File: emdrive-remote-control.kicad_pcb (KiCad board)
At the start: 2 copper layers, 107 x 46 mm, 43 parts, among them J1 Raspberry_Pi_2_3, J2 Screw_Terminal_01x06, J3 Conn_01x04, K1 Relay_SPST-NO, Q1 DMN61D8LQ, SW3 SW_Push, SW4 SW_Push, U1 ADS1015IDGS, U2 WS2801SO, U3 AP62150WU, U5 SN74HCS125, U6 MCP602, U7 BTS6143D

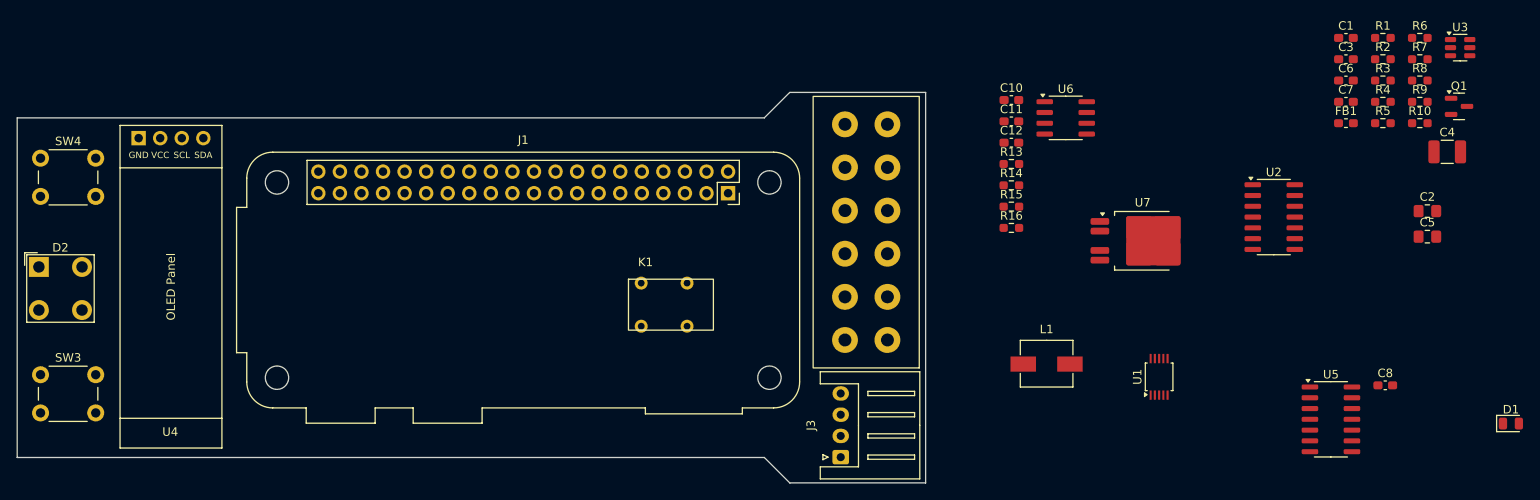
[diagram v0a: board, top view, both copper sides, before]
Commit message: Continues SCH, placed components on PCB
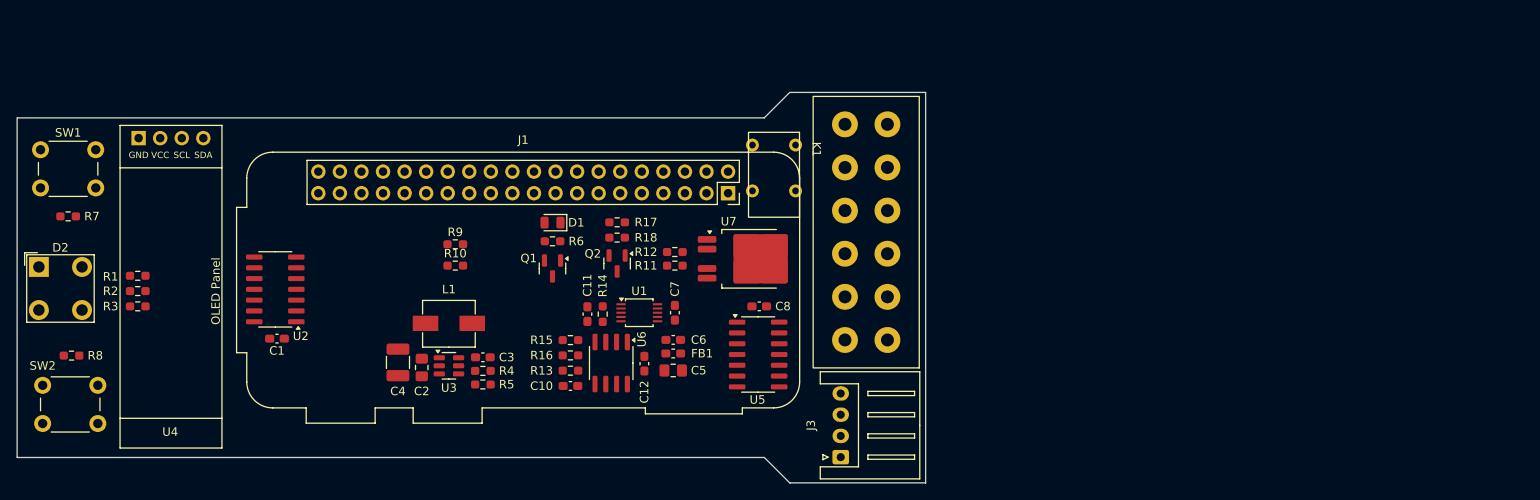
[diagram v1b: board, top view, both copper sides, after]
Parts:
- removed SW3, SW4: SW_Push, Button_Switch_THT:SW_PUSH_6mm_H8mm
- added Q2: MMBT3904, Package_TO_SOT_SMD:SOT-23, F.Cu at (149.7, 67.2)
- added R11: 33k, Resistor_SMD:R_0603_1608Metric_Pad0.98x0.95mm_HandSolder, F.Cu at (156.5, 67.4)
- added R12: 33k, Resistor_SMD:R_0603_1608Metric_Pad0.98x0.95mm_HandSolder, F.Cu at (156.5, 65.8)
- added R17: 33k, Resistor_SMD:R_0603_1608Metric_Pad0.98x0.95mm_HandSolder, F.Cu at (149.7, 62.3)
- added R18: 33k, Resistor_SMD:R_0603_1608Metric_Pad0.98x0.95mm_HandSolder, F.Cu at (149.7, 64.1)
- added SW1: SW_Push, Button_Switch_THT:SW_PUSH_6mm_H8mm, F.Cu at (81.8, 53.8)
- added SW2: SW_Push, Button_Switch_THT:SW_PUSH_6mm_H8mm, F.Cu at (82.0, 81.5)
- moved R8 162.1 mm to (85.4, 78.0)
- moved R7 160.3 mm to (85.0, 61.6)
- moved R1 149.3 mm to (93.2, 68.6), turned to 180 degrees
- moved R2 149.2 mm to (93.2, 70.4), turned to 180 degrees
- moved R3 149.1 mm to (93.2, 72.2), turned to 180 degrees
- moved C1 130.8 mm to (109.6, 76.0), turned to 180 degrees
- moved C4 126.1 mm to (123.8, 78.8), turned to 90 degrees
- moved U3 124.9 mm to (129.8, 79.2)
- moved C2 119.9 mm to (126.7, 79.4), turned to -90 degrees
- moved U2 117.9 mm to (109.4, 70.2), turned to 180 degrees
- moved D1 115.3 mm to (142.1, 62.3), turned to 180 degrees
- moved R10 114.8 mm to (130.6, 67.4)
- moved R9 114.8 mm to (130.6, 64.9)
- moved R4 110.6 mm to (133.8, 79.8), turned to 180 degrees
- moved R5 110.4 mm to (133.8, 81.4)
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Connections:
- C10 pad 1: GNDA -> GND
- C11 pad 1: GNDA -> GND
- C12 pad 1: GNDA -> GND
- C6 pad 1: GNDA -> GND
- J1 pad 1: Net-(J1-3V3-Pad1) -> +3.3V
- J1 pad 14: Net-(J1-GND-Pad14) -> GND
- J1 pad 15: unconnected-(J1-GPIO22-Pad15) -> /IN_LED_R
- J1 pad 16: unconnected-(J1-GPIO23-Pad16) -> /IN_LED_G
- J1 pad 17: Net-(J1-3V3-Pad1) -> +3.3V
- J1 pad 18: unconnected-(J1-GPIO24-Pad18) -> /IN_LED_Y
- J1 pad 19: unconnected-(J1-MOSI0/GPIO10-Pad19) -> /SPI_MOSI
- J1 pad 2: Net-(J1-5V-Pad2) -> +5V
- J1 pad 20: Net-(J1-GND-Pad14) -> GND
- J1 pad 23: unconnected-(J1-SCLK0/GPIO11-Pad23) -> /SPI_SCLK
- J1 pad 25: Net-(J1-GND-Pad14) -> GND
- J1 pad 26: unconnected-(J1-~{CE1}/GPIO7-Pad26) -> /WDT_EN
- J1 pad 29: unconnected-(J1-GCLK1/GPIO5-Pad29) -> /BTN_2
- J1 pad 3: unconnected-(J1-SDA/GPIO2-Pad3) -> /I2C_SDA
- J1 pad 30: Net-(J1-GND-Pad14) -> GND
- J1 pad 31: unconnected-(J1-GCLK2/GPIO6-Pad31) -> /DRIVE_PS_EN
- J1 pad 34: Net-(J1-GND-Pad14) -> GND
- J1 pad 39: Net-(J1-GND-Pad14) -> GND
- J1 pad 4: Net-(J1-5V-Pad2) -> +5V
- J1 pad 5: unconnected-(J1-SCL/GPIO3-Pad5) -> /I2C_SCL
- J1 pad 6: Net-(J1-GND-Pad14) -> GND
- J1 pad 7: unconnected-(J1-GCLK0/GPIO4-Pad7) -> /BTN_1
- J1 pad 9: Net-(J1-GND-Pad14) -> GND
- J2 pad 1: unconnected-(J2-Pin_1-Pad1) -> +12V
- J2 pad 2: unconnected-(J2-Pin_2-Pad2) -> GND
- J2 pad 3: unconnected-(J2-Pin_3-Pad3) -> Net-(J2-Pin_3)
- J2 pad 4: unconnected-(J2-Pin_4-Pad4) -> GND
- J2 pad 5: unconnected-(J2-Pin_5-Pad5) -> /WDT_P1
- J2 pad 6: unconnected-(J2-Pin_6-Pad6) -> /WDT_P2
- K1 pad 13: +12V -> /WDT_P2
- K1 pad 14: +12L -> /WDT_P1
- Q1 pad 1: Net-(Q1-G) -> /WDT_EN
- R10 pad 2: Net-(U1-SDA) -> /I2C_SDA
- R14 pad 2: unconnected-(R14-Pad2) -> /I_SENSE
- R16 pad 2: Net-(J4-Pin_4) -> GND
- R6 pad 2: Net-(Q1-G) -> /WDT_EN
- R7 pad 1: Net-(R7-Pad1) -> /BTN_1
- R8 pad 1: Net-(R8-Pad1) -> /BTN_2
- R9 pad 2: Net-(U1-SCL) -> /I2C_SCL
- U1 pad 1: GNDA -> GND
- U1 pad 10: Net-(U1-SCL) -> /I2C_SCL
- U1 pad 3: GNDA -> GND
- U1 pad 9: Net-(U1-SDA) -> /I2C_SDA
- U2 pad 1: unconnected-(U2-CKI-Pad1) -> /SPI_SCLK
- U2 pad 2: unconnected-(U2-SDI-Pad2) -> /SPI_MOSI
- U4 pad 3: Net-(U1-SCL) -> /I2C_SCL
- U4 pad 4: Net-(U1-SDA) -> /I2C_SDA
- U5 pad 3: unconnected-(U5-Y1-Pad3) -> /IN_LED_R
- U5 pad 6: unconnected-(U5-Y2-Pad6) -> /IN_LED_G
- U5 pad 8: unconnected-(U5-Y3-Pad8) -> /IN_LED_Y
- U6 pad 4: GNDA -> GND
- U7 pad 1: Net-(U7-OUT-Pad1) -> Net-(J2-Pin_3)
- U7 pad 2: unconnected-(U7-IN-Pad2) -> Net-(U7-IN)
- U7 pad 3: unconnected-(U7-Vbb-Pad3) -> +12V
- U7 pad 4: unconnected-(U7-IS-Pad4) -> /I_SENSE
- U7 pad 5: Net-(U7-OUT-Pad1) -> Net-(J2-Pin_3)
